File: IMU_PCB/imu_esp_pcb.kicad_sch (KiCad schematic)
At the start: 22 parts, among them J1 Conn_01x02_Pin, J2 Conn_01x05_Pin, U1 MPU-6050, U2 ESP32-C3-WROOM-02, U3 PTS647SM38SMTR2LFS, U4 XC6206P332MR-G, U5 1N5819HW-7-F

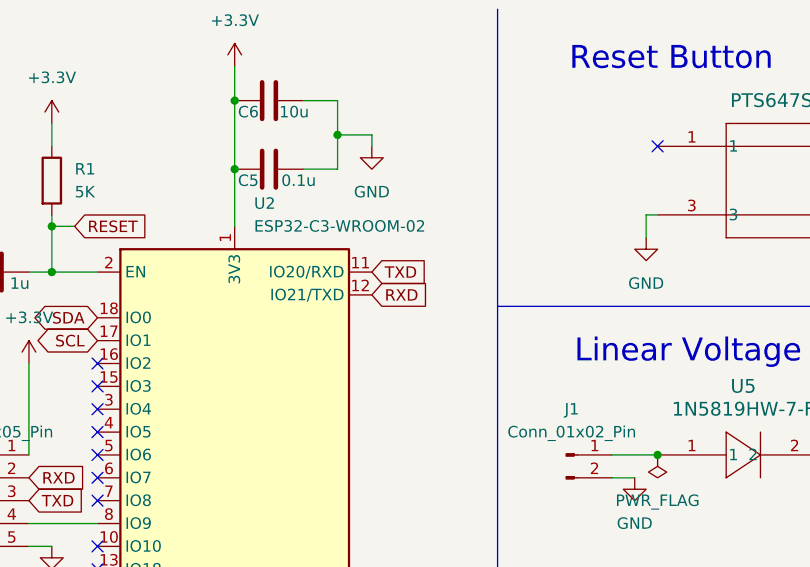
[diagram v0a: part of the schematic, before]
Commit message: Updated Schematic
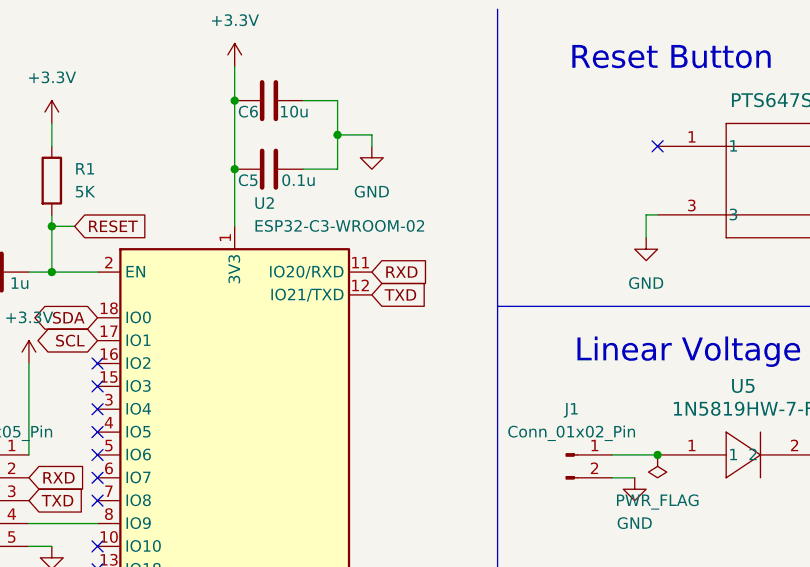
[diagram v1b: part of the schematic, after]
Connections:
- net RXD: now also U2.11 (IO20/RXD); no longer U2.12 (IO21/TXD)
- net TXD: now also U2.12 (IO21/TXD); no longer U2.11 (IO20/RXD)
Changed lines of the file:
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@@
 	(global_label "TXD"
 		(shape input)
-		(at 167.64 41.91 0)
+		(at 167.64 44.45 0)
 		(fields_autoplaced yes)
 		(effects
@@
 		)
 		(property "Intersheetrefs" "${INTERSHEET_REFS}"
-			(at 174.0723 41.91 0)
+			(at 174.0723 44.45 0)
 			(effects
 				(font
@@
 	(global_label "RXD"
 		(shape input)
-		(at 167.64 44.45 0)
+		(at 167.64 41.91 0)
 		(fields_autoplaced yes)
 		(effects
@@
 		)
 		(property "Intersheetrefs" "${INTERSHEET_REFS}"
-			(at 174.3747 44.45 0)
+			(at 174.3747 41.91 0)
 			(effects
 				(font
